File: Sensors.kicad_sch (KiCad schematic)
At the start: 15 parts, among them U19 BME280

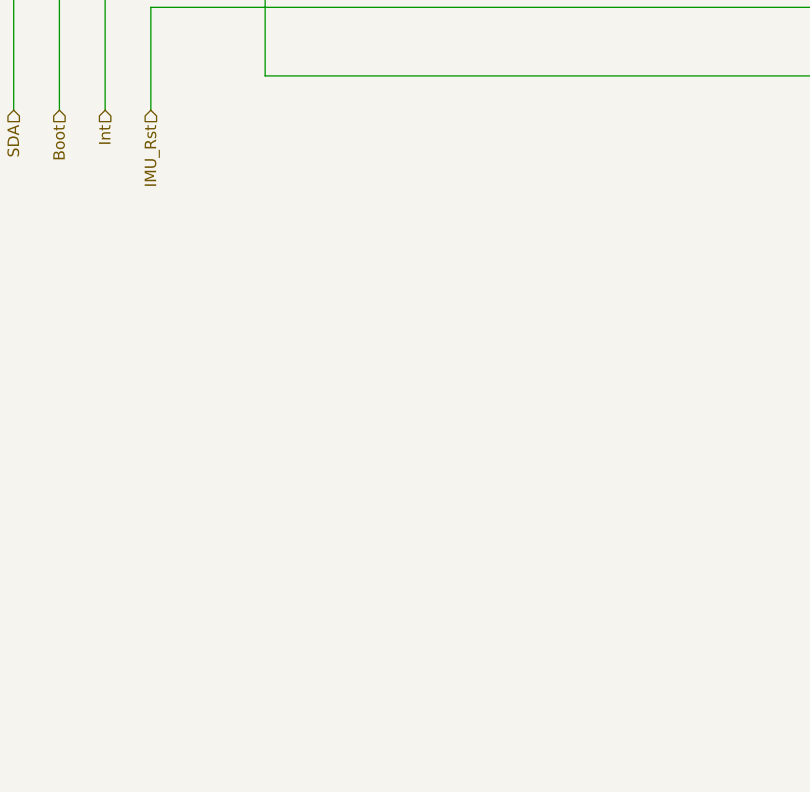
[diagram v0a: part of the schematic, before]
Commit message: stuff
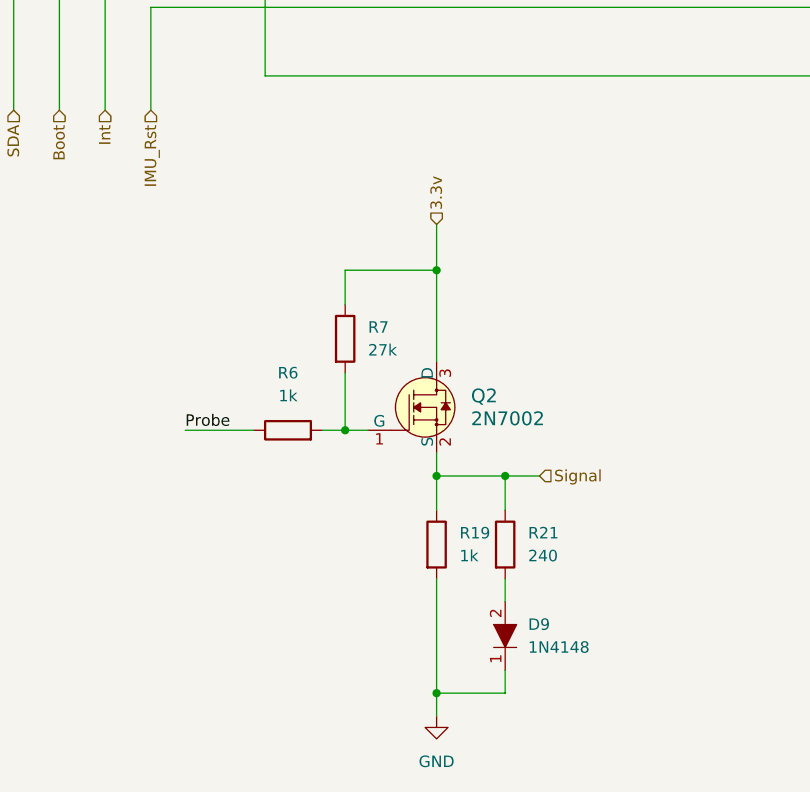
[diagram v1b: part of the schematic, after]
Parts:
- added D9: 1N4148, digikey-footprints:Diode_DO-35_P10mm, symbol dk_Diodes-Rectifiers-Single:1N4148
- added Q2: 2N7002, digikey-footprints:SOT-23-3, symbol dk_Transistors-FETs-MOSFETs-Single:2N7002
- added R19, R6: 1k, symbol Device:R
- added R21: 240, symbol Device:R
- added R7: 27k, symbol Device:R
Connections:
- net 3.3v: now also Q2.3 (D), R7.1
- net GND: now also D9.1, R19.2
- new net: Q2.1 (G), R6.2, R7.2
- new net: D9.2, R21.2
- new net Probe: R6.1
- new net Signal: Q2.2 (S), R19.1, R21.1
